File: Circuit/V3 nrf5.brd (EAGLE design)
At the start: 41 x 64.5 mm, 77 parts, among them J4 USB Micro, J7 CORTEX_DEBUG_SMD, Q1 FDV301N, Q2 BSS84, U1 AL8805, U2 MCP73831, U3 BC840M, U4 3.3V/150mA, U5 AL8805, U6 AL8805, U8 TPS61236P, Y1 32.768kHz

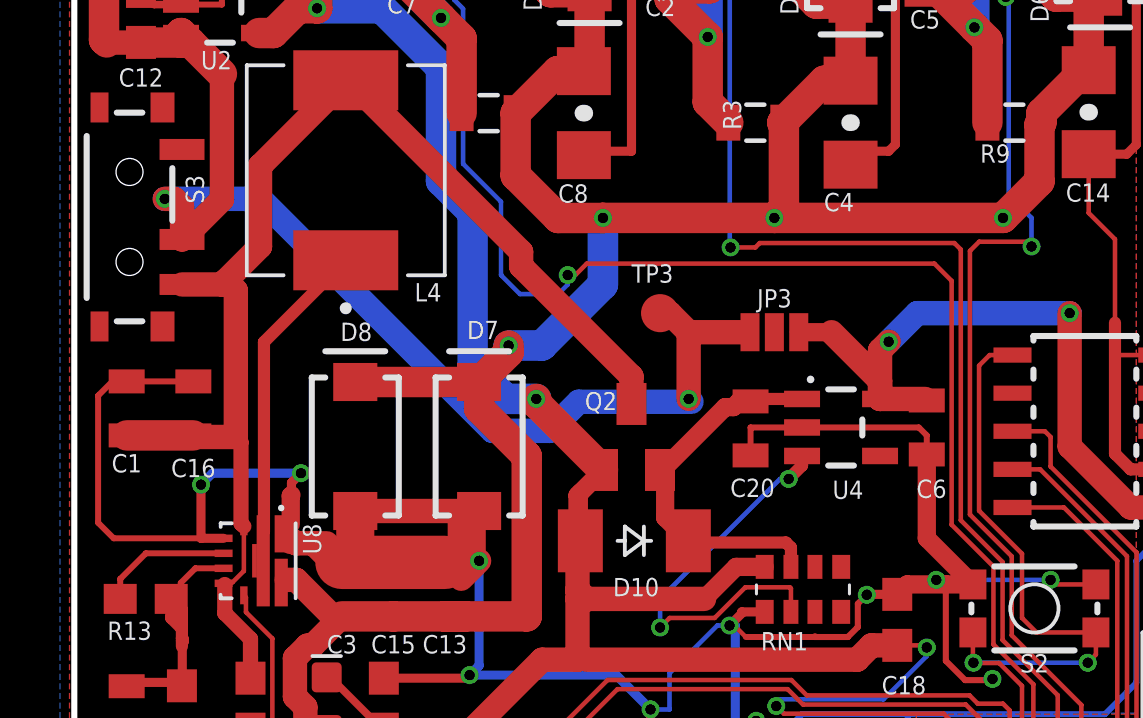
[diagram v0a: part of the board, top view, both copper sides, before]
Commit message: traces
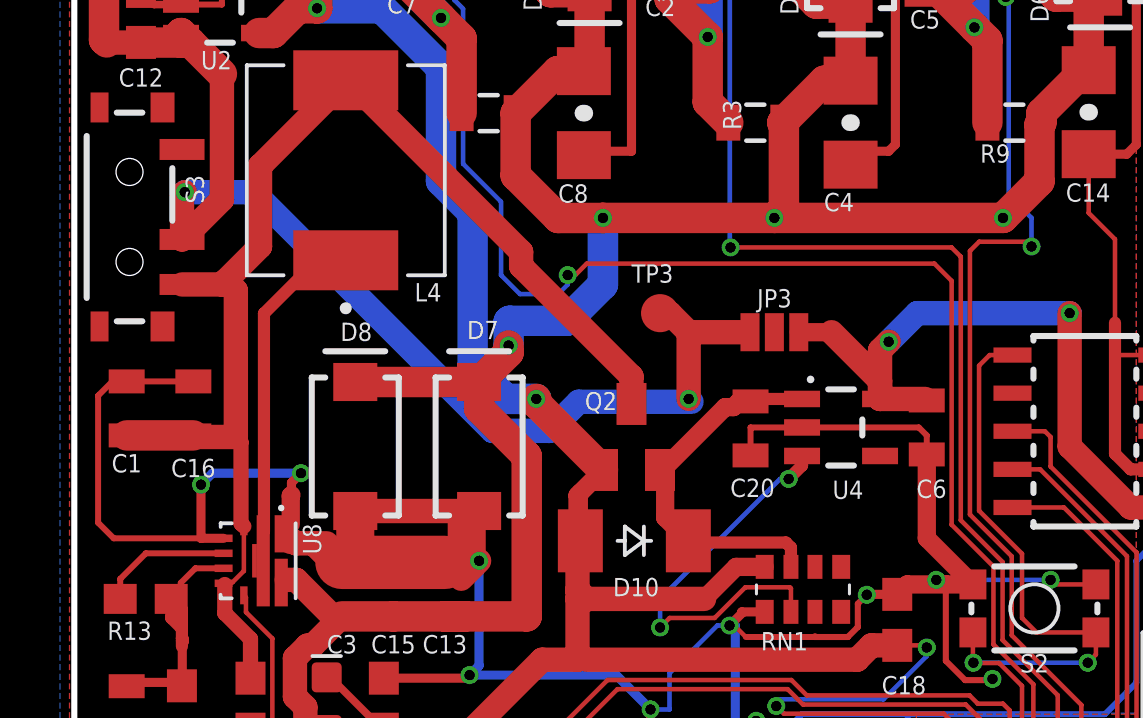
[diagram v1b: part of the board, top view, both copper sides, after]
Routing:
- net VBAT_S: track 65.4 -> 64.7 mm
- net N$3: track 12.8 -> 13.4 mm
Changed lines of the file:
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@@
 <via x="22.0345" y="35.21075" extent="1-16" drill="0.35"/>
 <wire x1="22.0091" y1="35.23615" x2="22.0345" y2="35.21075" width="0.1524" layer="16"/>
-<wire x1="23.00605" y1="35.3568" x2="22.86" y2="35.21075" width="0.1524" layer="1"/>
-<wire x1="22.0345" y1="35.21075" x2="22.86" y2="35.21075" width="0.1524" layer="1"/>
-<wire x1="23.00605" y1="35.3568" x2="29.49500625" y2="35.3568" width="0.1524" layer="1"/>
-<wire x1="29.49500625" y1="35.3568" x2="29.7084" y2="35.14340625" width="0.1524" layer="1"/>
+<wire x1="22.0345" y1="35.21075" x2="29.4005" y2="35.21075" width="0.1524" layer="1"/>
+<wire x1="29.4005" y1="35.21075" x2="29.7084" y2="34.90285" width="0.1524" layer="1"/>
+<wire x1="29.7084" y1="34.90285" x2="29.7084" y2="26.11794375" width="0.1524" layer="1"/>
 <wire x1="29.7084" y1="26.11794375" x2="31.1023" y2="24.72404375" width="0.1524" layer="1"/>
-<wire x1="29.7084" y1="35.14340625" x2="29.7084" y2="26.11794375" width="0.1524" layer="1"/>
 <wire x1="31.1023" y1="22.1230625" x2="31.1023" y2="24.72404375" width="0.1524" layer="1"/>
 <contactref element="U3" pad="A2"/>
@@
 <wire x1="3.7465" y1="18.8985" x2="2.109" y2="18.8985" width="0.8128" layer="1"/>
 <via x="14.63675" y="31.9405" extent="1-16" drill="0.35"/>
-<wire x1="17.78" y1="33.9725" x2="15.748" y2="31.9405" width="1.016" layer="16"/>
-<wire x1="14.63675" y1="31.9405" x2="15.748" y2="31.9405" width="1.016" layer="16"/>
+<wire x1="17.78" y1="33.9725" x2="16.5735" y2="32.766" width="1.016" layer="16"/>
+<wire x1="14.63675" y1="31.9405" x2="14.63675" y2="32.73425" width="1.016" layer="16"/>
+<wire x1="14.6685" y1="32.766" x2="14.63675" y2="32.73425" width="1.016" layer="16"/>
+<wire x1="16.5735" y1="32.766" x2="14.6685" y2="32.766" width="1.016" layer="16"/>
 <wire x1="17.78" y1="33.9725" x2="17.78" y2="36.195" width="1.016" layer="16"/>
 <via x="17.78" y="36.195" extent="1-16" drill="0.35"/>
@@
 <wire x1="6.4565" y1="25.7175" x2="6.4565" y2="27.305" width="0.3048" layer="1"/>
 <wire x1="6.4565" y1="27.305" x2="6.5165" y2="27.365" width="0.3048" layer="1"/>
-<wire x1="9.2075" y1="34.7825" x2="6.4809" y2="32.0559" width="0.4064" layer="1"/>
+<wire x1="9.2075" y1="34.7825" x2="8.255" y2="34.7825" width="0.4064" layer="1"/>
+<wire x1="8.255" y1="34.7825" x2="6.4809" y2="33.0084" width="0.4064" layer="1"/>
 <wire x1="6.4809" y1="25.7419" x2="6.4565" y2="25.7175" width="0.4064" layer="1"/>
-<wire x1="6.4809" y1="32.0559" x2="6.4809" y2="25.7419" width="0.4064" layer="1"/>
+<wire x1="6.4809" y1="33.0084" x2="6.4809" y2="25.7419" width="0.4064" layer="1"/>
 </signal>
 <signal name="N$8">
@@
 <wire x1="1.1494" y1="42.13490625" x2="1.24480625" y2="42.0395" width="0.8128" layer="1"/>
 <wire x1="1.24480625" y1="42.0395" x2="2.386" y2="42.0395" width="0.8128" layer="1"/>
-<wire x1="3.75025" y1="35.47675" x2="3.75025" y2="36.57225" width="0.8128" layer="1"/>
-<wire x1="3.75025" y1="36.57225" x2="3.4925" y2="36.83" width="0.8128" layer="1"/>
-<wire x1="3.4925" y1="36.83" x2="3.175" y2="36.83" width="0.8128" layer="1"/>
-<via x="3.175" y="36.83" extent="1-16" drill="0.35"/>
+<wire x1="3.84175" y1="37.05225" x2="3.75025" y2="36.96075" width="0.8128" layer="1"/>
+<wire x1="3.75025" y1="36.96075" x2="3.75025" y2="35.47675" width="0.8128" layer="1"/>
+<via x="3.84175" y="37.05225" extent="1-16" drill="0.35"/>
 <wire x1="14.09824375" y1="29.0957" x2="15.9993875" y2="29.0957" width="0.8128" layer="16"/>
-<wire x1="3.175" y1="36.83" x2="6.36394375" y2="36.83" width="0.8128" layer="16"/>
+<wire x1="3.84175" y1="37.05225" x2="6.14169375" y2="37.05225" width="0.8128" layer="16"/>
 <wire x1="16.9709375" y1="30.06725" x2="20.73275" y2="30.06725" width="0.8128" layer="16"/>
-<wire x1="6.36394375" y1="36.83" x2="14.09824375" y2="29.0957" width="0.8128" layer="16"/>
+<wire x1="6.14169375" y1="37.05225" x2="14.09824375" y2="29.0957" width="0.8128" layer="16"/>
 <wire x1="15.9993875" y1="29.0957" x2="16.9709375" y2="30.06725" width="0.8128" layer="16"/>
 <wire x1="20.6375" y1="32.385" x2="20.6375" y2="30.1625" width="0.8128" layer="1"/>
